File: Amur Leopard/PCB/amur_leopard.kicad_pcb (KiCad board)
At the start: 2 copper layers, 110.3 x 38.1 mm, 32 parts, among them SW1 SW_Push, U1 ATmega32U4-AU, Y1 16MHz

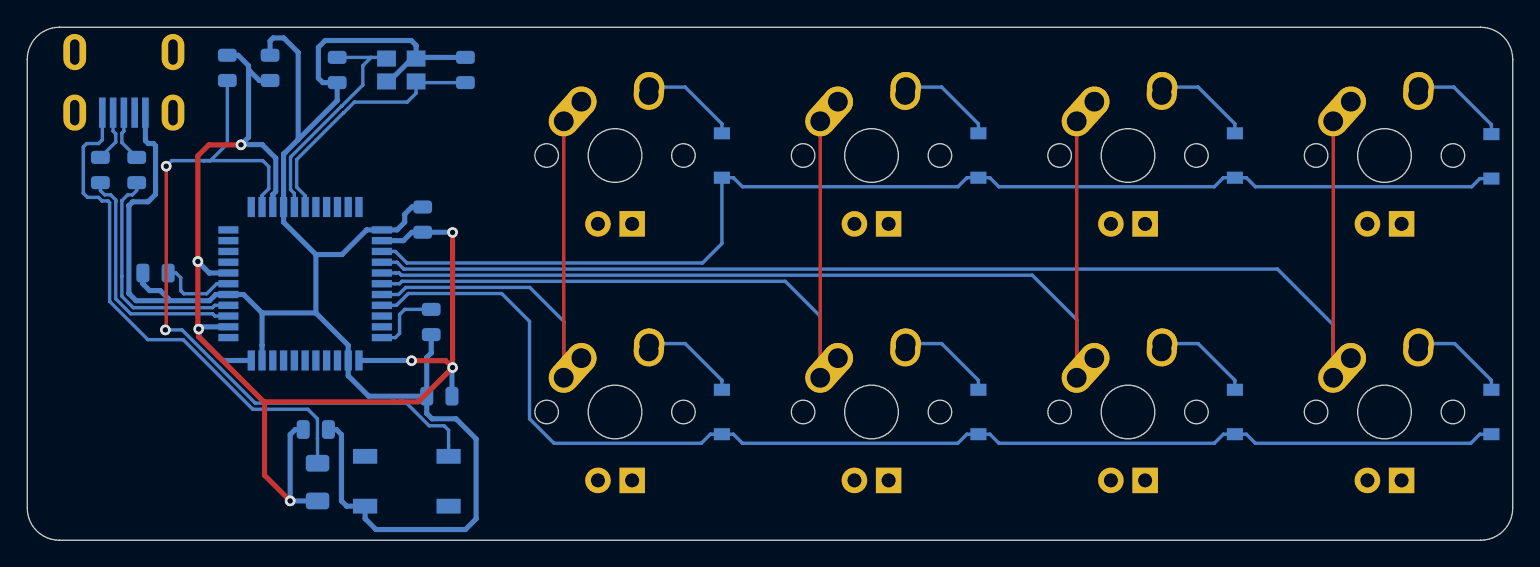
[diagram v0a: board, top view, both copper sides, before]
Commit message: Improve Amur Leopard-PCB
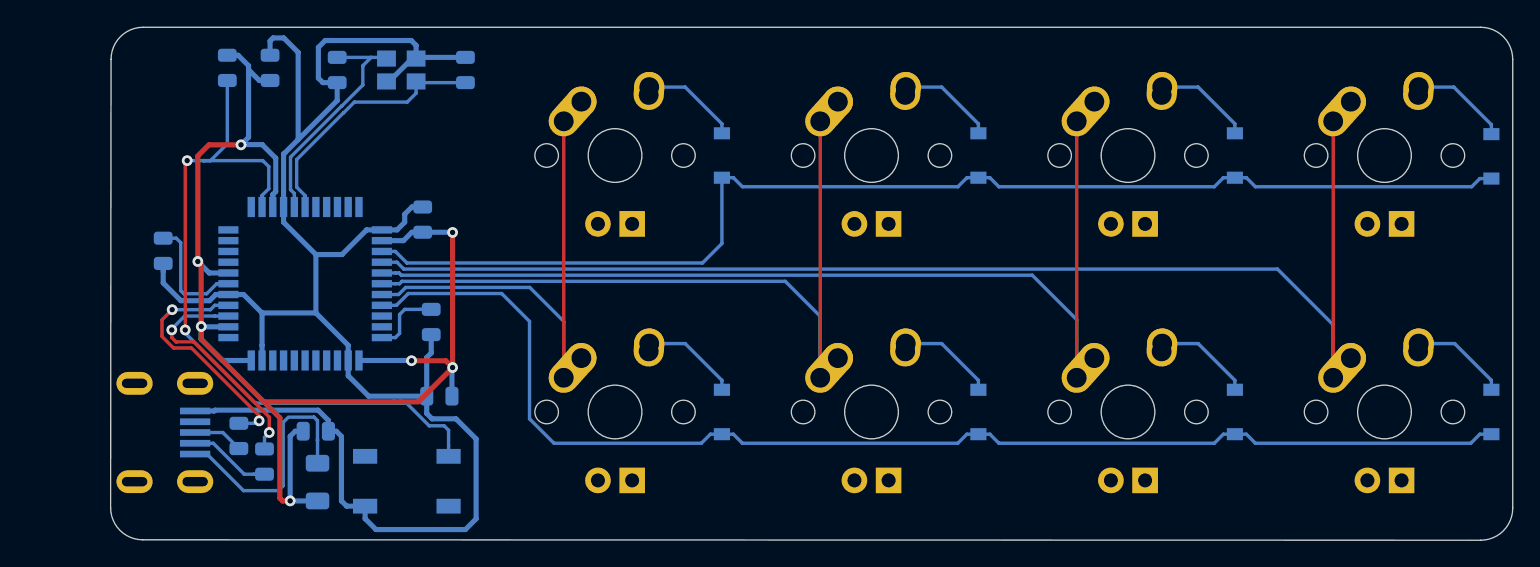
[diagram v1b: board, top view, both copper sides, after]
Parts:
- moved USB1 28.3 mm to (151.6, 109.5), turned to 0 degrees
- moved R3 24.8 mm to (161.3, 111.6), turned to 270 degrees
- moved R2 21.2 mm to (159.4, 109.7), turned to 270 degrees
- moved C3 1.75 mm to (153.8, 96.0), turned to 270 degrees
- moved C7 0.13 mm to (165.1, 109.4)
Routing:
- net VCC: track 39.0 -> 18.5 mm
- net GND: track 142.3 -> 133.6 mm
- net Net-(C3-Pad1): track 5.98 -> 8.94 mm
- net Net-(R1-Pad2): track 56.4 -> 53.8 mm
- net D-: track 3.88 -> 6.10 mm
- net Net-(R3-Pad1): track 18.3 -> 17.4 mm, vias 0 -> 2
- net Net-(R2-Pad1): track 17.4 -> 18.2 mm, vias 0 -> 2
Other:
- board size 110.3 x 38.1 mm -> 104.1 x 38.1 mm
